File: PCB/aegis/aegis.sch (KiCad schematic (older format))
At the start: 106 parts, among them Q1 TIP120, U1 ProMicro

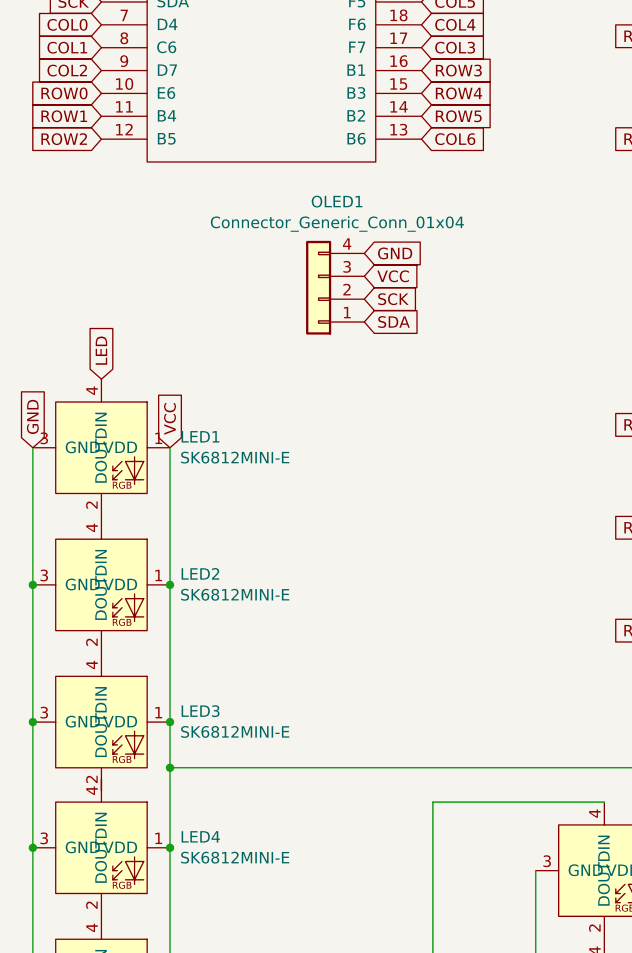
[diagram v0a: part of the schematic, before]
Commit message: save
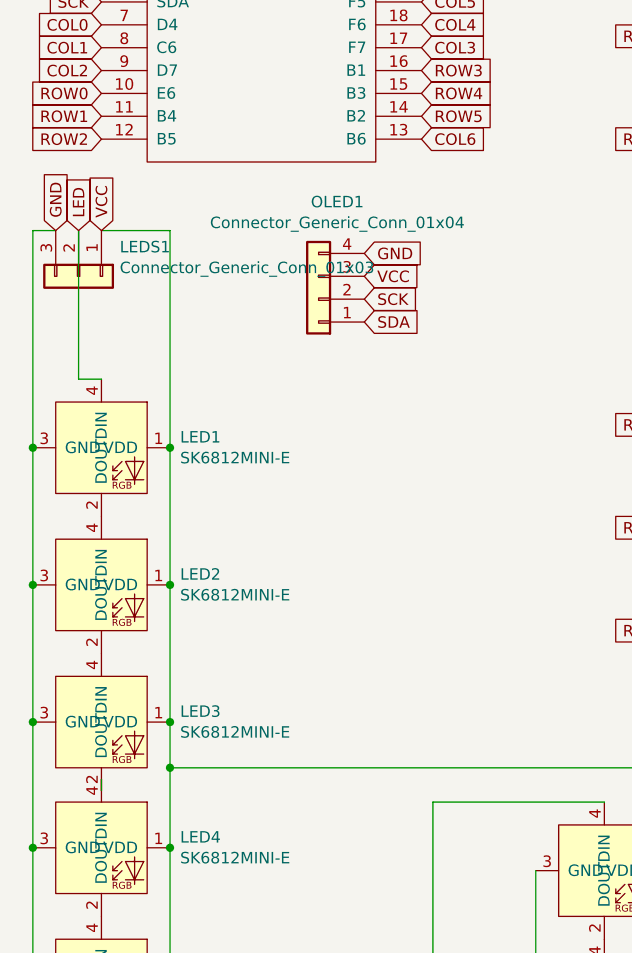
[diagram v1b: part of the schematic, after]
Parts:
- added LEDS1: Connector_Generic_Conn_01x03, Connector:FanPinHeader_1x03_P2.54mm_Vertical, symbol corne-classic-cache:Connector_Generic_Conn_01x03
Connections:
- net GND: now also LEDS1.3 (Pin_3)
- net LED: now also LEDS1.2 (Pin_2)
- net VCC: now also LEDS1.1 (Pin_1)
- net at LED3.2 (DOUT): now also LED4.4 (DIN)
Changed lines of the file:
@@
 SDA
-$Comp
-L SK6812MINI-E:SK6812MINI-E LED1
-U 1 1 5F95B6F7
-P 1150 3850
-F 0 "LED1" H 1494 3896 50  0000 L CNN
-F 1 "SK6812MINI-E" H 1494 3805 50  0000 L CNN
-F 2 "footprints:INV-YS-SK6812MINI-" H 1500 3650 50  0001 C CNN
-F 3 "" H 1500 3650 50  0001 C CNN
-	1    1150 3850
-	1    0    0    -1
-$EndComp
 $Comp
 L SK6812MINI-E:SK6812MINI-E LED2
@@
 	1    0    0    -1
 $EndComp
-Text GLabel 1450 3850 1    50   Input ~ 0
+Text GLabel 1150 2900 1    50   Input ~ 0
 VCC
-Text GLabel 850  3850 1    50   Input ~ 0
+Text GLabel 950  2900 1    50   Input ~ 0
 GND
-Text GLabel 1150 3550 1    50   Input ~ 0
+Text GLabel 1050 2900 1    50   Input ~ 0
 LED
 Wire Wire Line
@@
 Wire Wire Line
 	9800 3500 9950 3500
+$Comp
+L corne-classic-cache:Connector_Generic_Conn_01x03 LEDS1
+U 1 1 5FA19415
+P 1050 3100
+F 0 "LEDS1" V 922 3280 50  0000 L CNN
+F 1 "Connector_Generic_Conn_01x03" V 1013 3280 50  0000 L CNN
+F 2 "Connector:FanPinHeader_1x03_P2.54mm_Vertical" H 1050 3100 50  0001 C CNN
+F 3 "" H 1050 3100 50  0001 C CNN
+	1    1050 3100
+	0    1    1    0
+$EndComp
+$Comp
+L SK6812MINI-E:SK6812MINI-E LED1
+U 1 1 5F95B6F7
+P 1150 3850
+F 0 "LED1" H 1494 3896 50  0000 L CNN
+F 1 "SK6812MINI-E" H 1494 3805 50  0000 L CNN
+F 2 "footprints:INV-YS-SK6812MINI-" H 1500 3650 50  0001 C CNN
+F 3 "" H 1500 3650 50  0001 C CNN
+	1    1150 3850
+	1    0    0    -1
+$EndComp
+Wire Wire Line
+	950  2900 850  2900
+Wire Wire Line
+	850  2900 850  3850
+Connection ~ 850  3850
+Wire Wire Line
+	1050 2900 1050 3550
+Wire Wire Line
+	1050 3550 1150 3550
+Wire Wire Line
+	1150 2900 1450 2900
+Wire Wire Line
+	1450 2900 1450 3850
+Connection ~ 1450 3850
+Wire Wire Line
+	1150 5300 1150 5350
 $EndSCHEMATC

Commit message: update
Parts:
- Solenoide1: footprint Connector_PinHeader_1.00mm:PinHeader_1x02_P1.00mm_Vertical -> Connector_PinHeader_1.27mm:PinHeader_1x02_P1.27mm_Horizontal
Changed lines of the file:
@@
 F 0 "Solenoide1" V 9245 2950 50  0000 C CNN
 F 1 "Motor_DC" V 9154 2950 50  0000 C CNN
-F 2 "Connector_PinHeader_1.00mm:PinHeader_1x02_P1.00mm_Vertical" H 8950 2910 50  0001 C CNN
+F 2 "Connector_PinHeader_1.27mm:PinHeader_1x02_P1.27mm_Horizontal" H 8950 2910 50  0001 C CNN
 F 3 "~" H 8950 2910 50  0001 C CNN
 	1    8950 3000
